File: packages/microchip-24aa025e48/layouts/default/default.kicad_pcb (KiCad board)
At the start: 2 copper layers, 4 parts

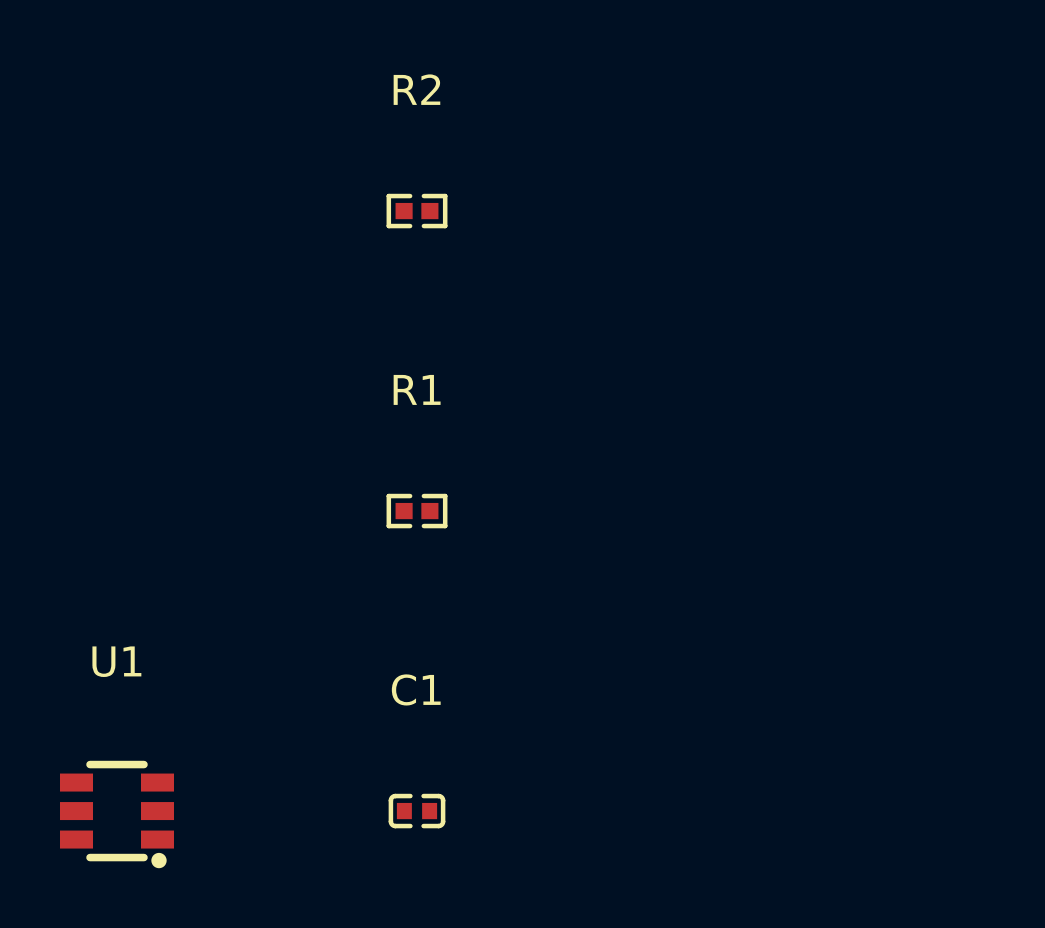
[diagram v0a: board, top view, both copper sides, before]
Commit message: Layout modules
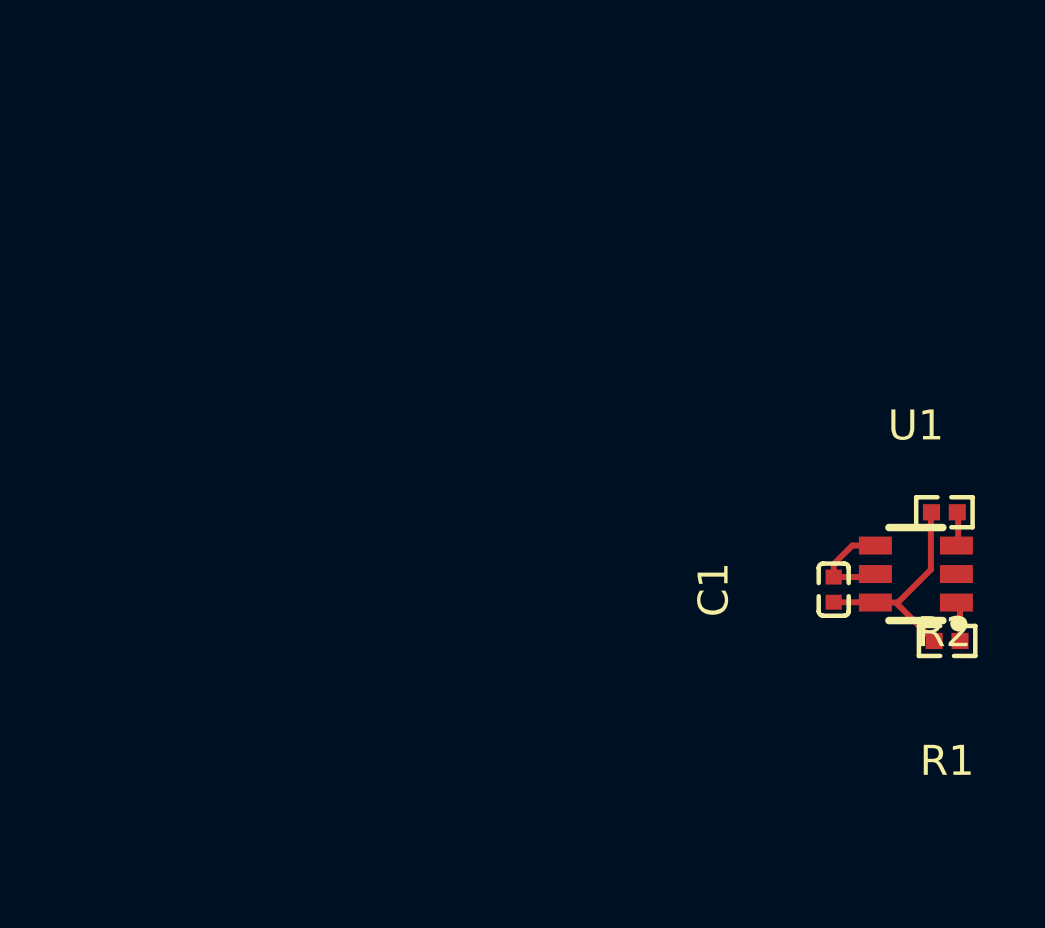
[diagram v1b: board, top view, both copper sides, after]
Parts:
- moved U1 27.8 mm to (26.6, -7.90)
- moved R2 20.2 mm to (27.6, -9.96), turned to 180 degrees
- moved R1 18.2 mm to (27.7, -5.67), turned to 180 degrees
- moved C1 15.7 mm to (23.9, -7.38), turned to 90 degrees
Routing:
- net hv: track 0.00 -> 7.37 mm
- net lv: track 0.00 -> 3.51 mm
- net SCL: track 0.00 -> 1.33 mm
- net SDA: track 0.00 -> 1.15 mm
